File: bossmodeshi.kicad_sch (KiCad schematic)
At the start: 102 parts, among them Q1 FZT853TA, Q2 PSMN3R7-100BSE, Q3 PSMN3R7-100BSE, Q4 PSMN3R7-100BSE, Q5 PSMN3R7-100BSE, U10 SQ1464EEH-T1_GE3, U11 MP2790DFP-0000-T, U5 SQ1464EEH-T1_GE3, U6 SQ1464EEH-T1_GE3, U7 SQ1464EEH-T1_GE3, U8 SQ1464EEH-T1_GE3, U9 SQ1464EEH-T1_GE3

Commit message: Did a lot of routing
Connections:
- net TOP: no longer R_CHG_PUP1.2
- net at D_CHG_VGS1.1 (K), R_CHG_DRIVER1.2, R_CHG_MG1.2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: no longer R_CHG_PUP1.1
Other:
- moved on the sheet: R_CHG_PUP1
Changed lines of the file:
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@@
 		(lib_id "Device:R")
 		(at 245.11 245.11 0)
+		(mirror y)
 		(unit 1)
 		(exclude_from_sim no)
@@
 		(dnp no)
 		(property "Reference" "R_SRN_FLT1"
-			(at 251.968 243.84 0)
+			(at 238.252 243.84 0)
 			(effects
 				(font
@@
 		)
 		(property "Value" "100"
-			(at 251.968 246.38 0)
+			(at 238.252 246.38 0)
 			(effects
 				(font
@@
 		)
 		(property "Footprint" "Resistor_SMD:R_0603_1608Metric"
-			(at 243.332 245.11 90)
+			(at 246.888 245.11 90)
 			(effects
 				(font
@@
 	(symbol
 		(lib_id "Device:R")
-		(at 213.36 41.91 180)
+		(at 356.87 -287.02 180)
 		(unit 1)
 		(exclude_from_sim no)
@@
 		(dnp no)
 		(property "Reference" "R_CHG_PUP1"
-			(at 208.788 40.132 90)
+			(at 352.298 -288.798 90)
 			(effects
 				(font
@@
 		)
 		(property "Value" "10 MΩ"
-			(at 210.82 40.894 90)
+			(at 354.33 -288.036 90)
 			(effects
 				(font
@@
 		)
 		(property "Footprint" "Resistor_SMD:R_0603_1608Metric"
-			(at 215.138 41.91 90)
+			(at 358.648 -287.02 90)
 			(effects
 				(font
@@
 		)
 		(property "Datasheet" "https://www.koaspeer.com/pdfs/RK73H.pdf"
-			(at 213.36 41.91 0)
+			(at 356.87 -287.02 0)
 			(effects
 				(font
@@
 		)
 		(property "Description" "RES 10M OHM 1% 1/10W 0402"
-			(at 213.36 41.91 0)
+			(at 356.87 -287.02 0)
 			(effects
 				(font
@@
 		)
 		(property "Mfr" "KOA Speer Electronics, Inc."
-			(at 213.36 41.91 0)
+			(at 356.87 -287.02 0)
 			(effects
 				(font
@@
 		)
 		(property "Mfr P/N" "RK73H1ETTP1005F"
-			(at 213.36 41.91 0)
+			(at 356.87 -287.02 0)
 			(effects
 				(font
@@
 		)
 		(property "Supplier_1" "Digikey"
-			(at 213.36 41.91 90)
+			(at 356.87 -287.02 90)
 			(effects
 				(font
@@
 		)
 		(property "Supplier_1 P/N" "2019-RK73H1ETTP1005FTR-ND"
-			(at 213.36 41.91 90)
+			(at 356.87 -287.02 90)
 			(effects
 				(font
@@
 		)
 		(property "Supplier_1 Price @ QTY" "1"
-			(at 213.36 41.91 90)
+			(at 356.87 -287.02 90)
 			(effects
 				(font
@@
 		)
 		(property "Supplier_1 Unit Price" "0.10000"
-			(at 213.36 41.91 90)
+			(at 356.87 -287.02 90)
 			(effects
 				(font
@@
 		)
 		(property "Supplier_2" ""
-			(at 213.36 41.91 90)
+			(at 356.87 -287.02 90)
 			(effects
 				(font
@@
 		)
 		(property "Supplier_2 P/N" ""
-			(at 213.36 41.91 90)
+			(at 356.87 -287.02 90)
 			(effects
 				(font
@@
 		)
 		(property "Supplier_2 Price @ QTY" ""
-			(at 213.36 41.91 90)
+			(at 356.87 -287.02 90)
 			(effects
 				(font
@@
 		)
 		(property "Supplier_2 Unit Price" ""
-			(at 213.36 41.91 90)
+			(at 356.87 -287.02 90)
 			(effects
 				(font
@@
 		)
 		(property "Supplier_1 Price @ Qty" ""
-			(at 213.36 41.91 0)
+			(at 356.87 -287.02 0)
 			(effects
 				(font
@@
 		)
 		(property "Supplier_2 Price @ Qty" ""
-			(at 213.36 41.91 0)
+			(at 356.87 -287.02 0)
 			(effects
 				(font

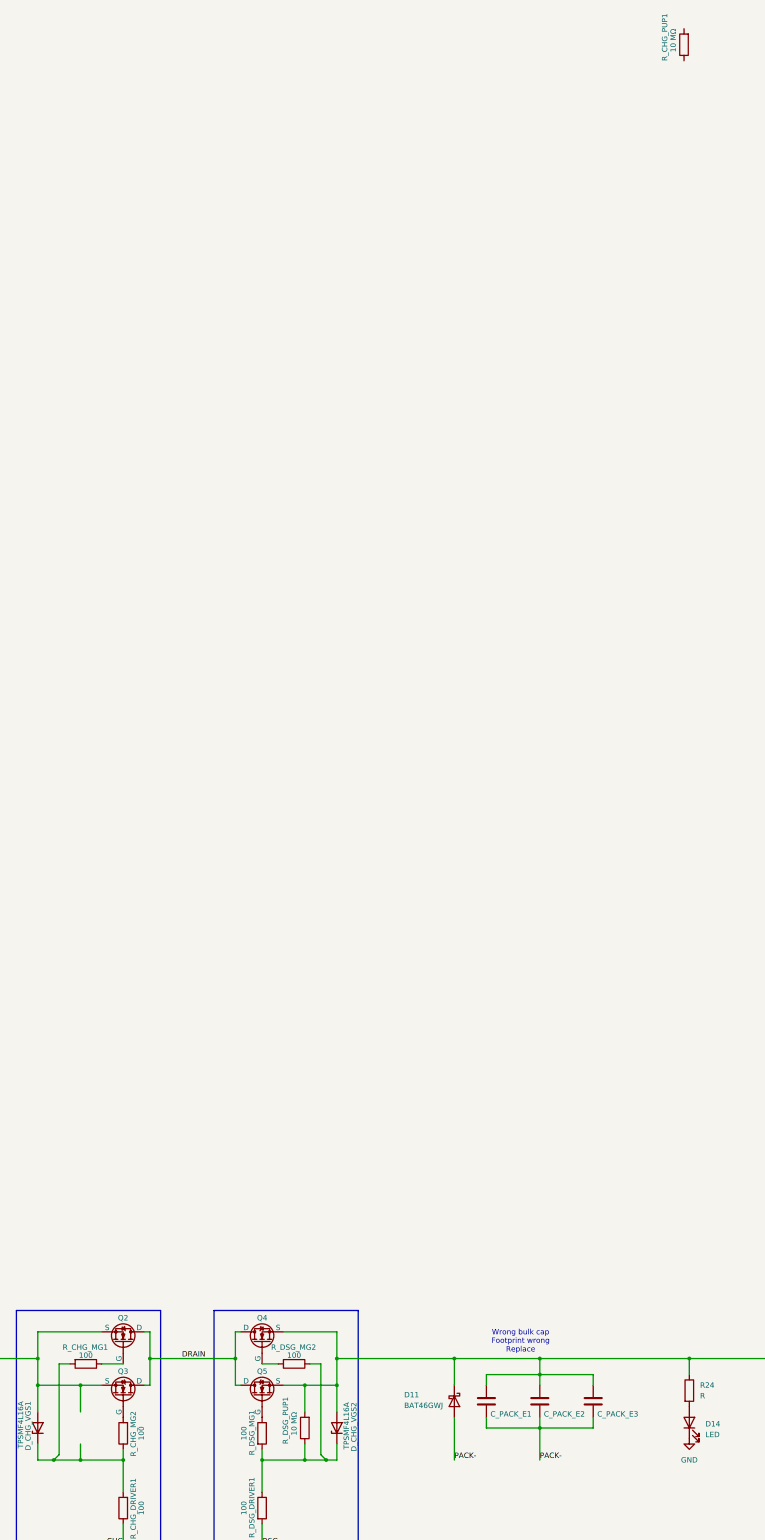
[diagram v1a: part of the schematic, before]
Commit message: Working on routing
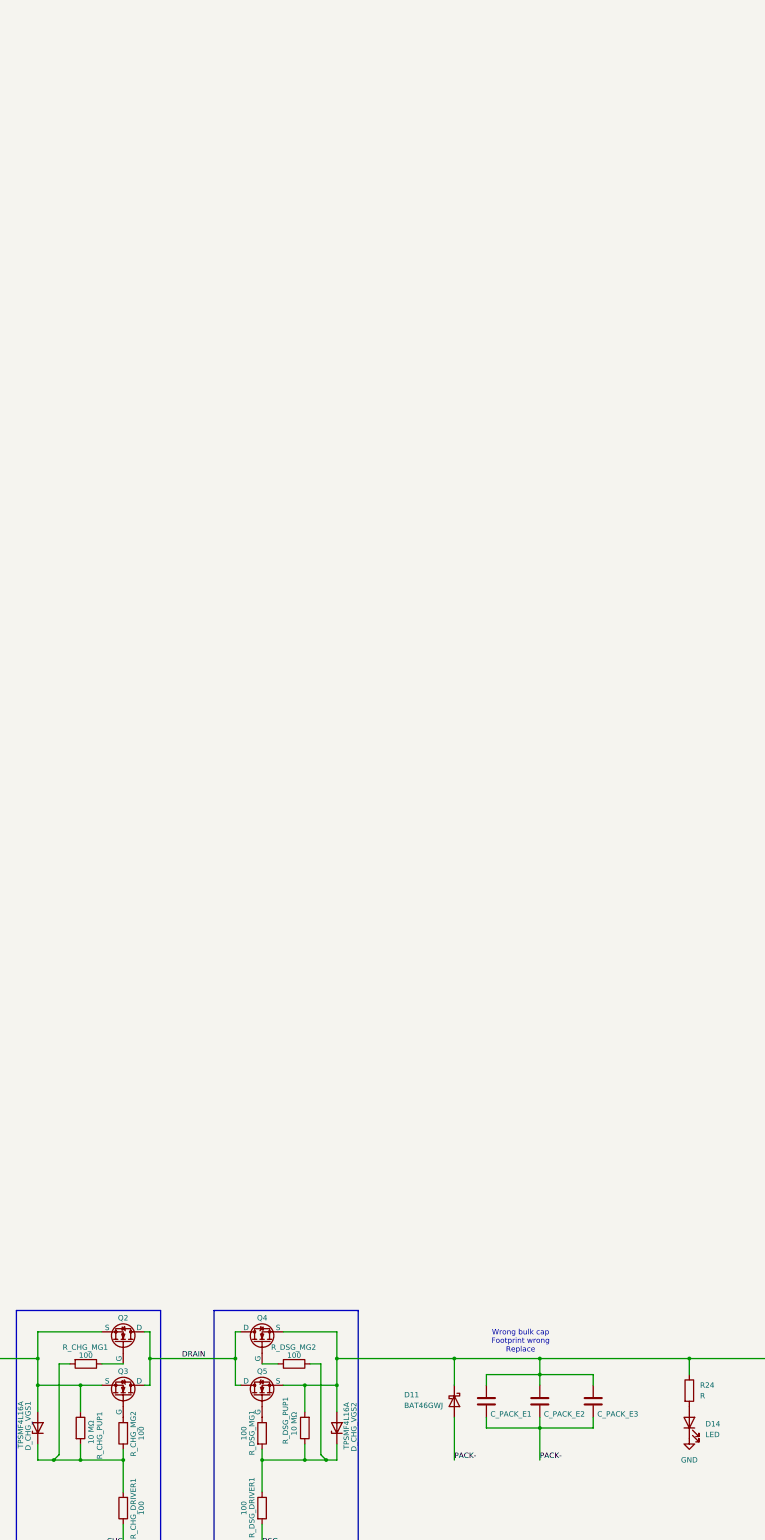
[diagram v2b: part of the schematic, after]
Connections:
- net TOP: now also R_CHG_PUP1.1
- net at D_CHG_VGS1.1 (K), R_CHG_DRIVER1.2, R_CHG_MG1.2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: now also R_CHG_PUP1.2
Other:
- moved on the sheet: R_CHG_PUP1
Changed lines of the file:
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@@
 	)
 	(symbol
-		(lib_name "SQ1464EEH-T1_GE3_1")
 		(lib_id "_SQ1464:SQ1464EEH-T1_GE3")
 		(at 64.77 228.6 0)
@@
 	)
 	(symbol
-		(lib_name "SQ1464EEH-T1_GE3_1")
 		(lib_id "_SQ1464:SQ1464EEH-T1_GE3")
 		(at 64.77 194.31 0)
@@
 	)
 	(symbol
-		(lib_name "SQ1464EEH-T1_GE3_1")
 		(lib_id "_SQ1464:SQ1464EEH-T1_GE3")
 		(at 64.77 160.02 0)
@@
 	)
 	(symbol
-		(lib_name "SQ1464EEH-T1_GE3_1")
 		(lib_id "_SQ1464:SQ1464EEH-T1_GE3")
 		(at 64.77 91.44 0)
@@
 	(symbol
 		(lib_id "Device:R")
-		(at 356.87 -287.02 180)
+		(at 213.36 41.91 0)
 		(unit 1)
 		(exclude_from_sim no)
@@
 		(dnp no)
 		(property "Reference" "R_CHG_PUP1"
-			(at 352.298 -288.798 90)
+			(at 217.932 43.688 90)
 			(effects
 				(font
@@
 		)
 		(property "Value" "10 MΩ"
-			(at 354.33 -288.036 90)
+			(at 215.9 42.926 90)
 			(effects
 				(font
@@
 		)
 		(property "Footprint" "Resistor_SMD:R_0603_1608Metric"
-			(at 358.648 -287.02 90)
+			(at 211.582 41.91 90)
 			(effects
 				(font
@@
 		)
 		(property "Datasheet" "https://www.koaspeer.com/pdfs/RK73H.pdf"
-			(at 356.87 -287.02 0)
+			(at 213.36 41.91 0)
 			(effects
 				(font
@@
 		)
 		(property "Description" "RES 10M OHM 1% 1/10W 0402"
-			(at 356.87 -287.02 0)
+			(at 213.36 41.91 0)
 			(effects
 				(font
@@
 		)
 		(property "Mfr" "KOA Speer Electronics, Inc."
-			(at 356.87 -287.02 0)
+			(at 213.36 41.91 0)
 			(effects
 				(font
@@
 		)
 		(property "Mfr P/N" "RK73H1ETTP1005F"
-			(at 356.87 -287.02 0)
+			(at 213.36 41.91 0)
 			(effects
 				(font
@@
 		)
 		(property "Supplier_1" "Digikey"
-			(at 356.87 -287.02 90)
+			(at 213.36 41.91 90)
 			(effects
 				(font
@@
 		)
 		(property "Supplier_1 P/N" "2019-RK73H1ETTP1005FTR-ND"
-			(at 356.87 -287.02 90)
+			(at 213.36 41.91 90)
 			(effects
 				(font
@@
 		)
 		(property "Supplier_1 Price @ QTY" "1"
-			(at 356.87 -287.02 90)
+			(at 213.36 41.91 90)
 			(effects
 				(font
@@
 		)
 		(property "Supplier_1 Unit Price" "0.10000"
-			(at 356.87 -287.02 90)
+			(at 213.36 41.91 90)
 			(effects
 				(font
@@
 		)
 		(property "Supplier_2" ""
-			(at 356.87 -287.02 90)
+			(at 213.36 41.91 90)
 			(effects
 				(font
@@
 		)
 		(property "Supplier_2 P/N" ""
-			(at 356.87 -287.02 90)
+			(at 213.36 41.91 90)
 			(effects
 				(font
@@
 		)
 		(property "Supplier_2 Price @ QTY" ""
-			(at 356.87 -287.02 90)
+			(at 213.36 41.91 90)
 			(effects
 				(font
@@
 		)
 		(property "Supplier_2 Unit Price" ""
-			(at 356.87 -287.02 90)
+			(at 213.36 41.91 90)
 			(effects
 				(font
@@
 		)
 		(property "Supplier_1 Price @ Qty" ""
-			(at 356.87 -287.02 0)
+			(at 213.36 41.91 0)
 			(effects
 				(font
@@
 		)
 		(property "Supplier_2 Price @ Qty" ""
-			(at 356.87 -287.02 0)
+			(at 213.36 41.91 0)
 			(effects
 				(font
@@
 	)
 	(symbol
-		(lib_name "SQ1464EEH-T1_GE3_1")
 		(lib_id "_SQ1464:SQ1464EEH-T1_GE3")
 		(at 64.77 57.15 0)
@@
 	)
 	(symbol
-		(lib_name "SQ1464EEH-T1_GE3_1")
 		(lib_id "_SQ1464:SQ1464EEH-T1_GE3")
 		(at 64.77 125.73 0)
